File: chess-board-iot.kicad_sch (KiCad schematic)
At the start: 58 parts

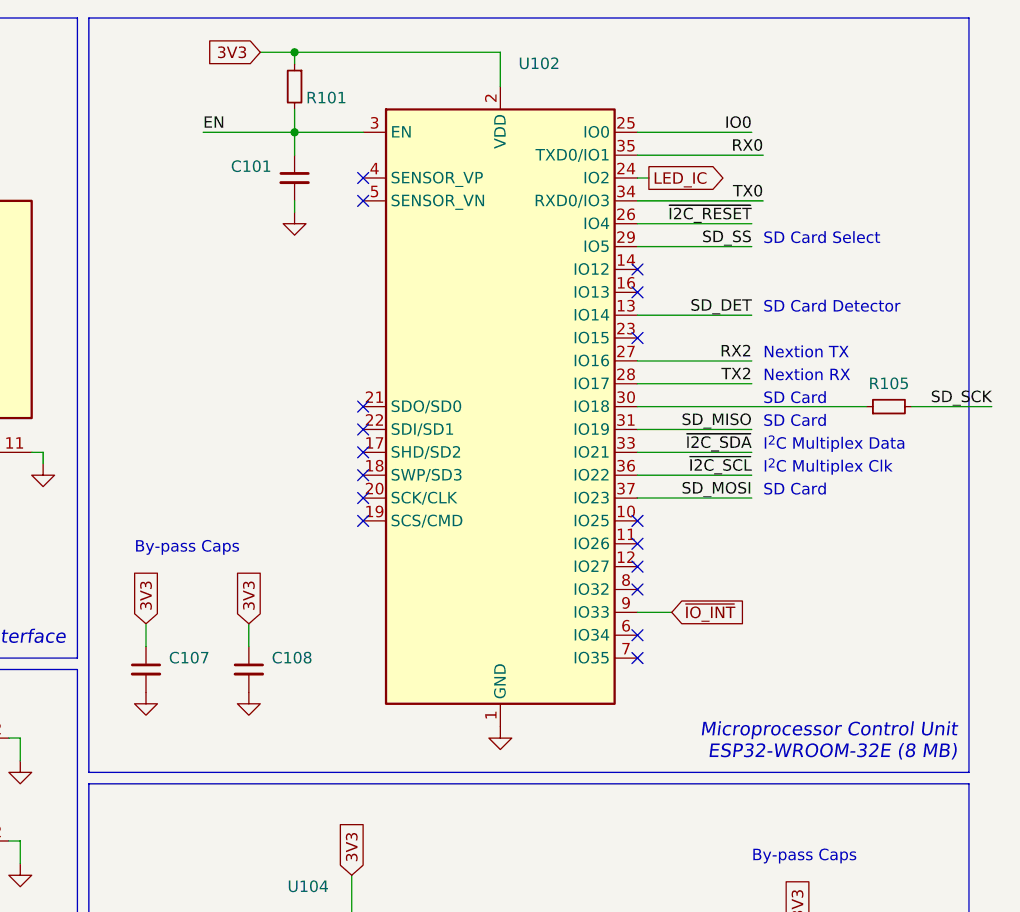
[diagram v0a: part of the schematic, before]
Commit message: fix sd card layout
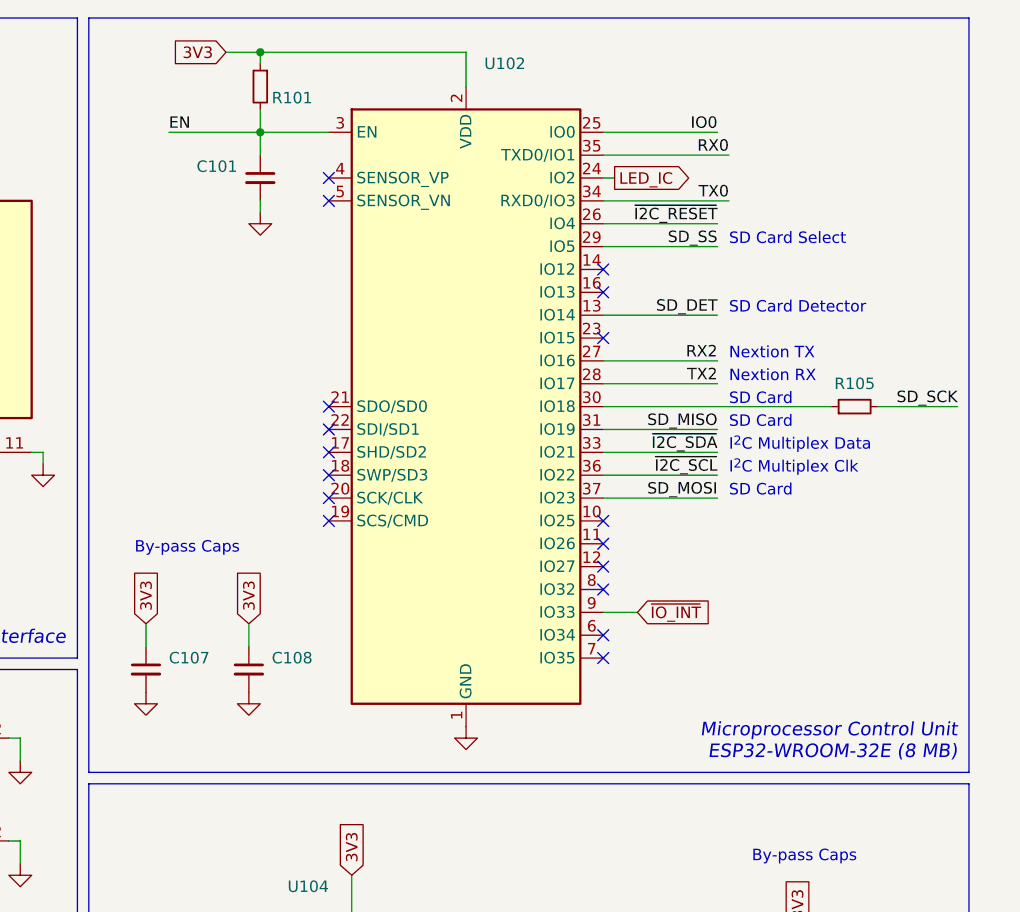
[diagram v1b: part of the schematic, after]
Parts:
- R105: LCSC (none) -> C107701
- R113, R114: LCSC (none) -> C21190
- R115: LCSC (none) -> C23179
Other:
- moved on the sheet: C101, R101, R105, U102

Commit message: fix USB-C footprint and traces
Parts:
- U102: LCSC C701341 -> C701342
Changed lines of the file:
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@@
       (effects (font (size 1.27 1.27)) hide)
     )
-    (property "LCSC" "C701341" (id 4) (at 285.75 57.15 0)
+    (property "LCSC" "C701342" (id 4) (at 285.75 57.15 0)
       (effects (font (size 1.27 1.27)) hide)
     )
@@
     )
     (path "/582a69f8-5434-4554-917e-70d2bc28584c"
-      (reference "J101") (unit 1) (value "USB_C_Receptacle_USB2.0") (footprint "Connector_USB:USB_C_Receptacle_JAE_DX07S016JA1R1500")
+      (reference "J101") (unit 1) (value "USB_C_Receptacle_USB2.0") (footprint "User Custom Footprint:USB_C_Receptable_918-418K2023S40001")
     )
     (path "/64f954f3-8828-4c30-b54d-fa7a7ce114c2"
@@
     )
     (path "/7531744a-adfd-462a-a28f-135299bc08b0"
-      (reference "U102") (unit 1) (value "ESP32-WROOM-32E") (footprint "RF_Module:ESP32-WROOM-32")
+      (reference "U102") (unit 1) (value "ESP32-WROOM-32E (8MB)") (footprint "RF_Module:ESP32-WROOM-32")
     )
     (path "/bbc54aa5-5efc-46ea-83fa-f9acfbcc058f"
